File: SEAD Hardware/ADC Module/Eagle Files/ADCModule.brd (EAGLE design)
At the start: 44.9 x 48.9 mm, 49 parts, among them IC2 93-C46AST, U1 LP2989_DGK_8, X1 52885-0374

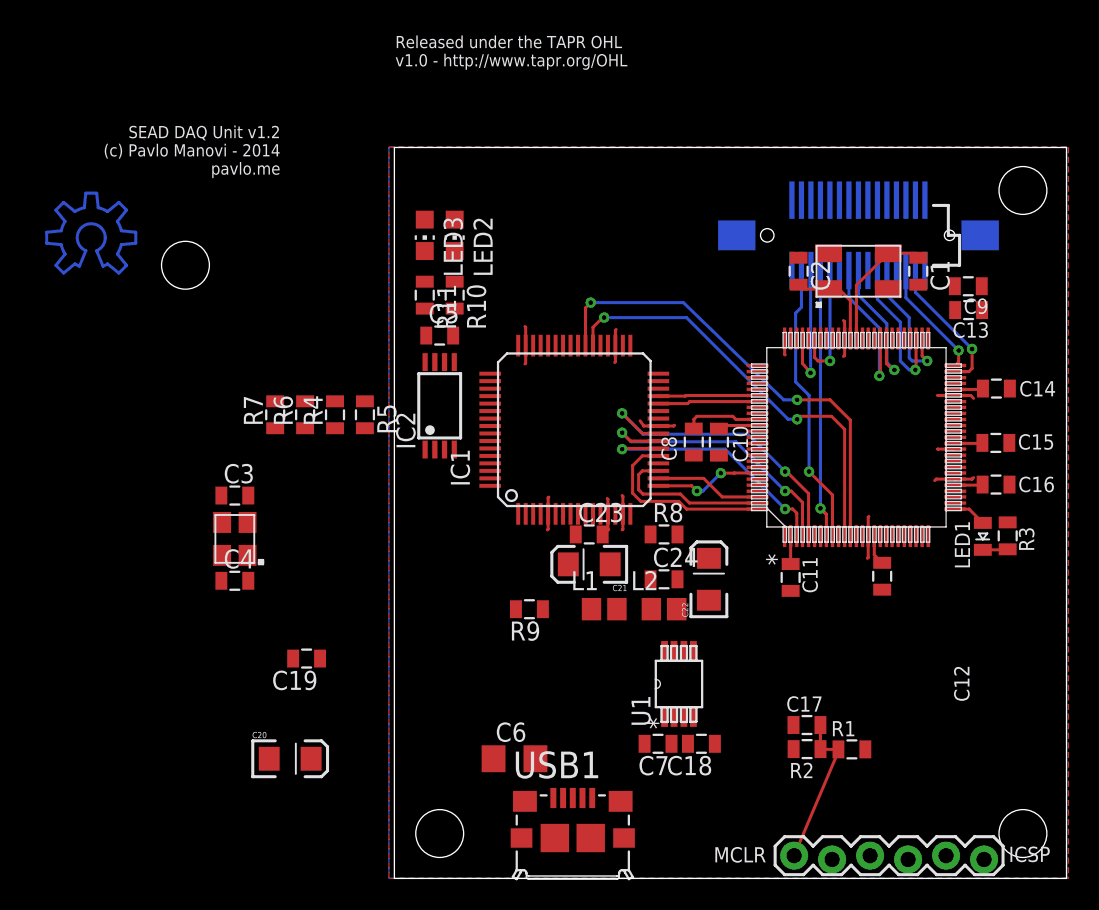
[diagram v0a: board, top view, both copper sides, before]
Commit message: More board layout work.
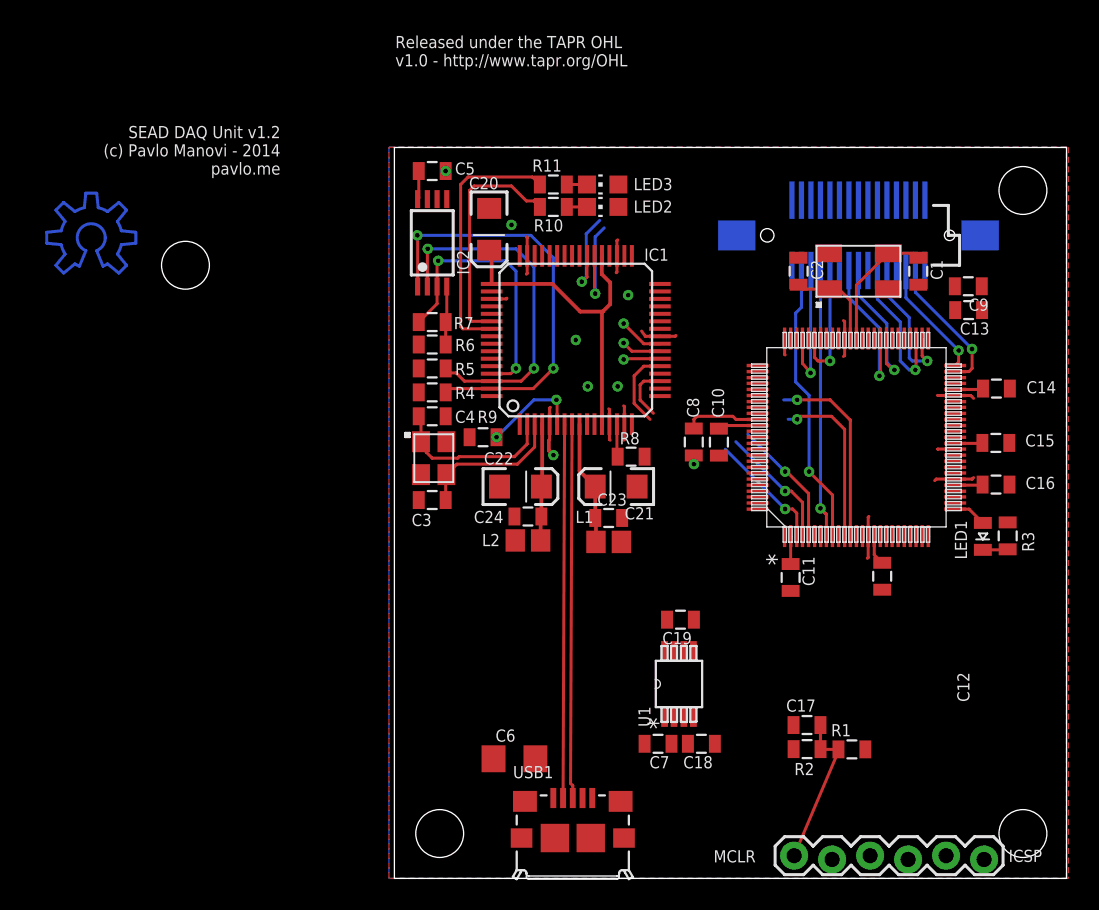
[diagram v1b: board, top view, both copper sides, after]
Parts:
- moved C20 37.8 mm to (6.30, 43.4), turned to 270 degrees
- moved C19 25.1 mm to (19.1, 17.3)
- moved C4 17.2 mm to (2.50, 30.9), turned to 180 degrees
- moved U$3 14.4 mm to (2.60, 28.1), turned to 270 degrees
- moved C22 14.0 mm to (8.40, 26.2), turned to 0 degrees
- moved C3 13.2 mm to (2.50, 25.3), turned to 180 degrees
- moved LED3 12.4 mm to (13.9, 46.4), turned to 90 degrees
- moved R7 12.2 mm to (2.50, 37.2), turned to 180 degrees
- moved R9 11.9 mm to (5.90, 29.5)
- moved R11 11.3 mm to (10.6, 46.4), turned to 180 degrees
- moved C5 11.0 mm to (2.50, 47.3)
- moved IC2 10.9 mm to (2.50, 42.5)
- moved L2 10.2 mm to (8.90, 22.6), turned to 180 degrees
- moved LED2 10.1 mm to (13.9, 44.9), turned to 90 degrees
- moved C24 10.0 mm to (8.90, 24.2), turned to 180 degrees
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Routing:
- net N$12: track 0.00 -> 28.6 mm, vias 0 -> 2
- net N$11: track 0.00 -> 25.1 mm
- net N$10: track 0.00 -> 25.0 mm
- net N$13: track 0.00 -> 23.5 mm, vias 0 -> 2
- net VDD1V8_D: track 0.00 -> 22.2 mm
- net N$18: track 0.00 -> 18.4 mm, vias 0 -> 2
- net N$29: track 0.00 -> 17.4 mm
- net N$28: track 0.00 -> 15.5 mm
- net USB_UART_RX: track 31.3 -> 19.3 mm
- net N$9: track 0.00 -> 11.2 mm
- net USB_UART_TX: track 28.7 -> 18.7 mm
- net N$8: track 0.00 -> 9.91 mm
- net D7: track 20.5 -> 11.5 mm
- net N$22: track 0.00 -> 8.33 mm
- net D6: track 18.9 -> 11.0 mm
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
